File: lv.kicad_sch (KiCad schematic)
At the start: 6 parts, among them J2 CAN_DEBUG_NANO_01x04, J3 CarLVPowerConnector, J4 CAN_NANO_01x05

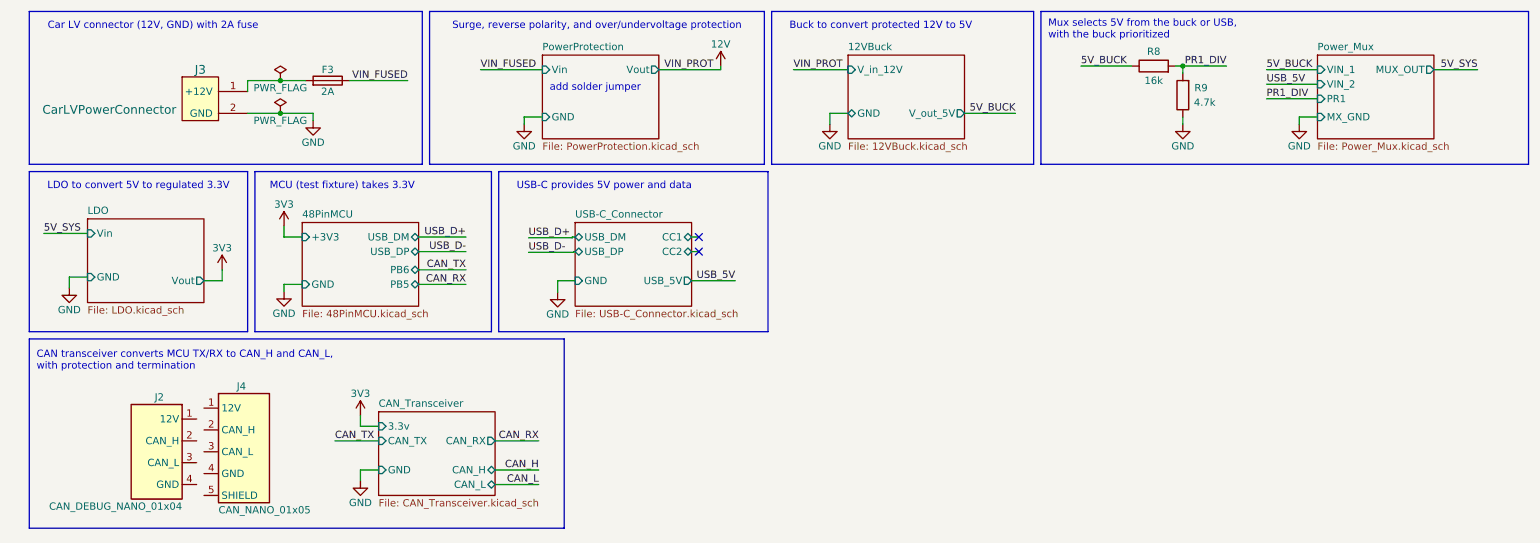
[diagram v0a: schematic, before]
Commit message: hv 1.3
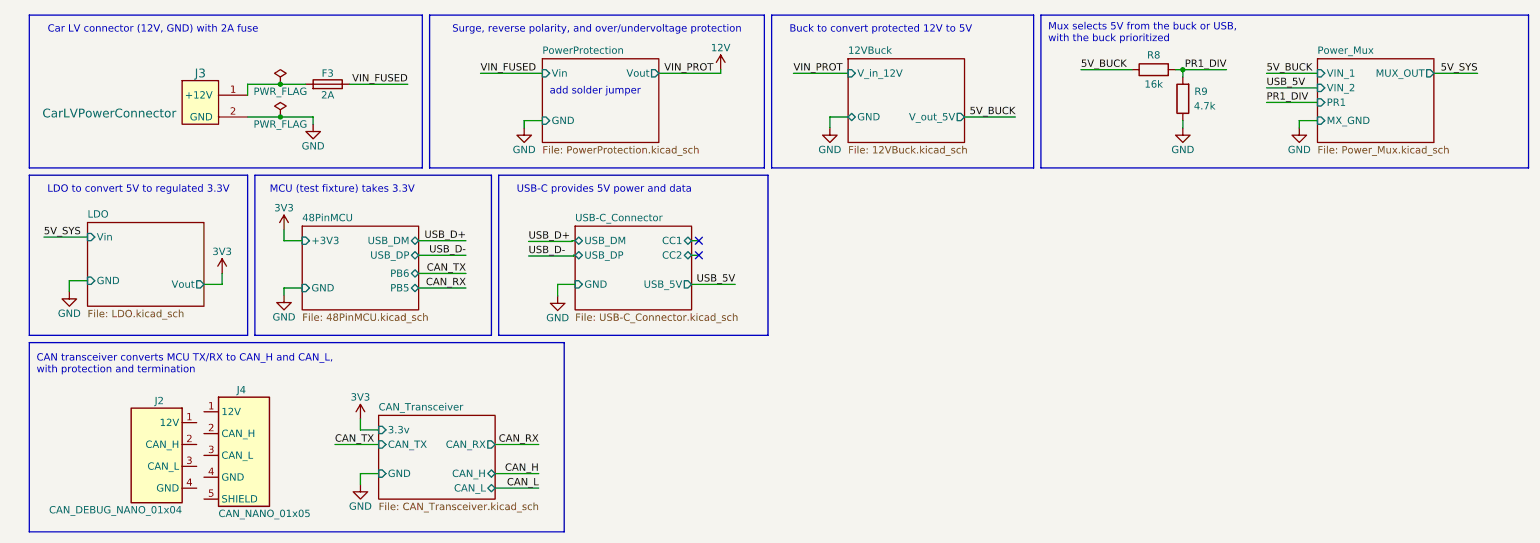
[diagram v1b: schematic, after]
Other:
- moved on the sheet: F3, J2, J3, J4, R8, R9
